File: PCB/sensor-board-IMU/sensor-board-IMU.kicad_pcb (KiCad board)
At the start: 2 copper layers, 20 x 20 mm, 6 parts, among them J2 Conn_01x03_Pin (data connecti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, J5 Conn_01x03_Pin (power connect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

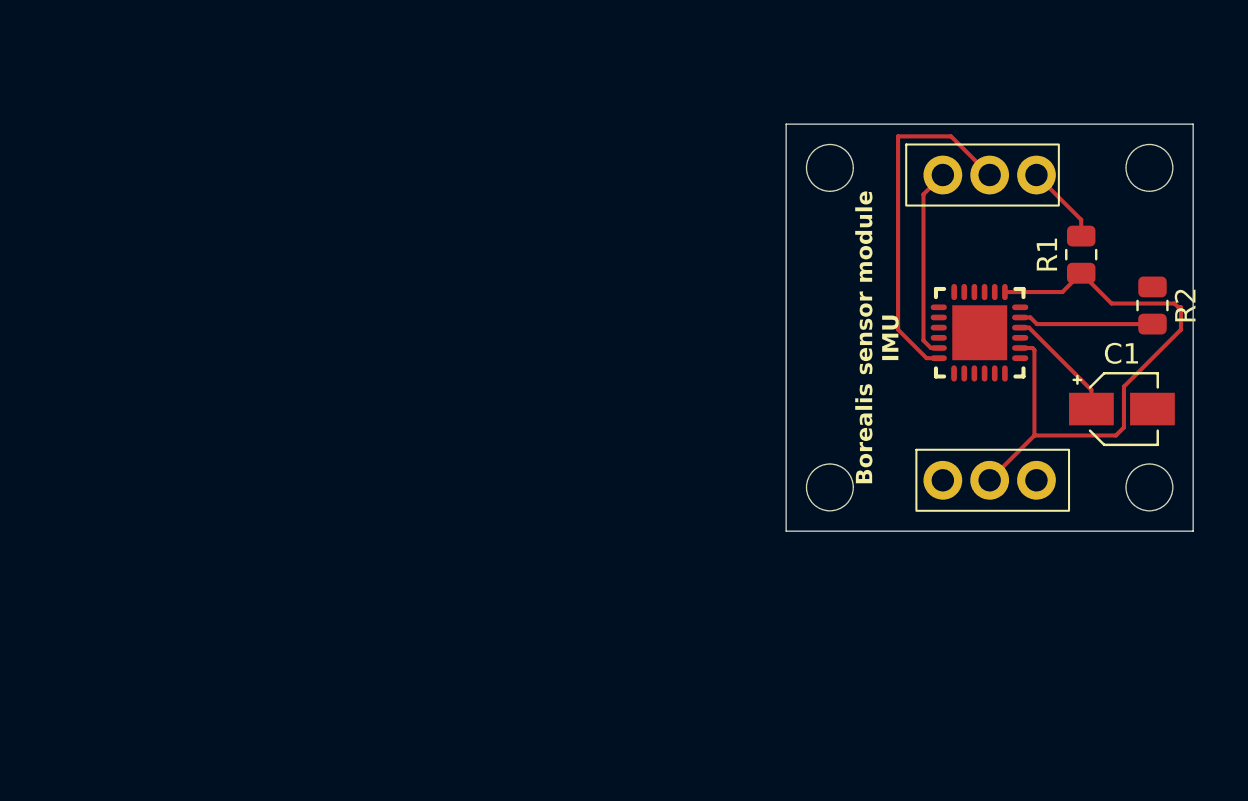
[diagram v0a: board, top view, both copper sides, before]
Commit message: Made some final checks and changes
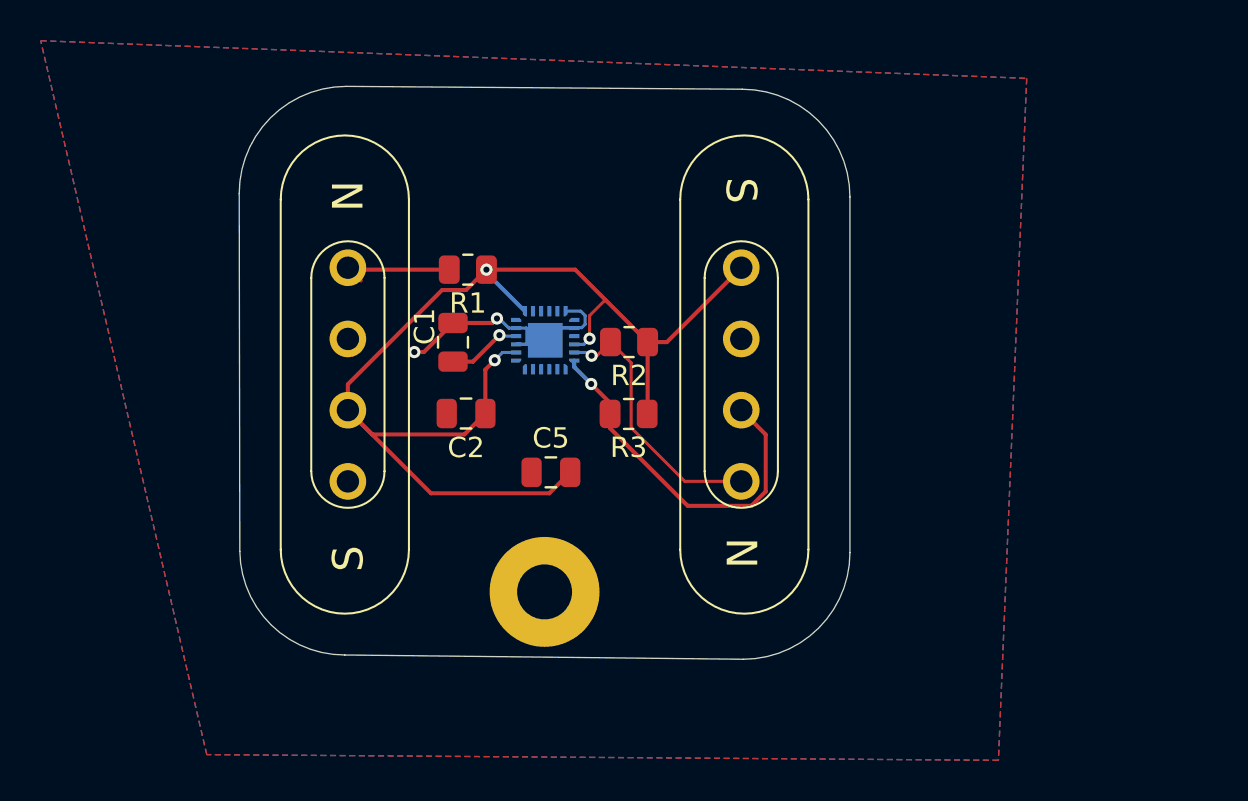
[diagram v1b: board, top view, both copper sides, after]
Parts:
- removed J2: Conn_01x03_Pin (data connection to main board), batteryholder:1x03 2.3 pitch
- removed J5: Conn_01x03_Pin (power connection to main board), batteryholder:1x03 2.3 pitch
- removed MPU6050: ~, batteryholder:MPU6050-footprint
- added C2: 10nF, Capacitor_SMD:C_0805_2012Metric, F.Cu at (89.8, 62.2)
- added C5: 0.1uf, Capacitor_SMD:C_0805_2012Metric, F.Cu at (93.9, 65.1)
- added G***: LOGO, LOGO, B.Cu at (93.9, 64.1)
- added H1: MountingHole, MountingHole:MountingHole_2.7mm_M2.5_Pad, F.Cu at (93.6, 71.0)
- added MPU6500: ~, batteryholder:mpu6500, B.Cu at (93.7, 58.6)
- added R3: 4.7k, Resistor_SMD:R_0805_2012Metric, F.Cu at (97.8, 62.2)
- added U1: MAGNETIC POGO CONN., batteryholder:MAGNETIC POGO CONN., F.Cu at (103.3, 60.3)
- added U2: MAGNETIC POGO CONN., batteryholder:MAGNETIC POGO CONN., F.Cu at (84.0, 60.3)
- C1: value 0.1 microf -> 0.1uF; footprint Capacitor_SMD:CP_Elec_3x5.3 -> Capacitor_SMD:C_0805_2012Metric
- R2: value 10k -> 4.7k
- moved C1 33.0 mm to (89.1, 58.7), turned to 90 degrees
- moved R1 30.1 mm to (89.9, 55.1), turned to 180 degrees
- moved R2 25.8 mm to (97.8, 58.7), turned to 180 degrees
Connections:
- R1 pad 2: /ADC -> /ID
- R2 pad 1: GND -> +3.3V
- R2 pad 2: Net-(MPU6050-AD0) -> /SCL
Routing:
- net +3.3V: track 29.4 -> 60.1 mm, vias 0 -> 3
- net GND: track 0.00 -> 14.7 mm, vias 0 -> 2
- net Net-(MPU6050-AD0): track 6.63 -> 0.00 mm
- net /ID: track 0.00 -> 5.91 mm
- net /ADC: track 3.91 -> 0.00 mm
- net /SCL: track 9.43 -> 13.3 mm, vias 0 -> 1
- net Net-(MPU6500-REGOUT): track 5.70 -> 3.66 mm, vias 0 -> 1
- net /SDA: track 17.4 -> 18.1 mm, vias 0 -> 1
- added copper zone on B.Cu, net GND
- added copper zone on F.Cu, net GND
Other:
- board size 20 x 20 mm -> 30 x 28.1 mm
- board text added: "BOREALIS"
- board text added: "INERTIAL MEASUREMENT UNIT"
- board text removed: "Borealis sensor module IMU"
